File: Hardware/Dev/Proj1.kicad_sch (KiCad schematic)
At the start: 4 parts, among them J1 Conn_01x02, SW1 SW_Push

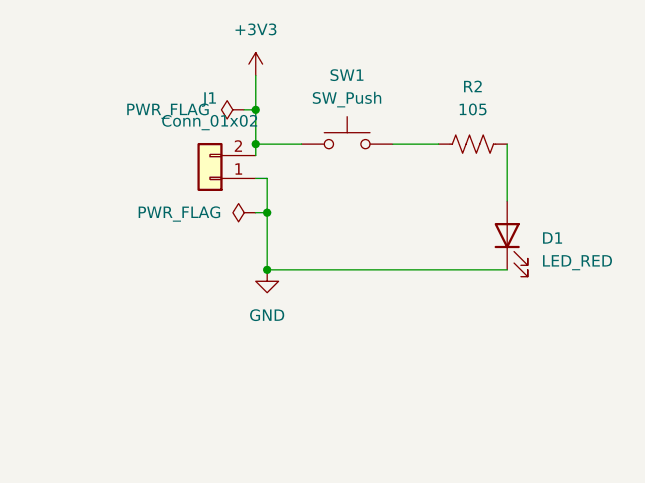
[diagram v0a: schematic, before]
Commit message: onboarding
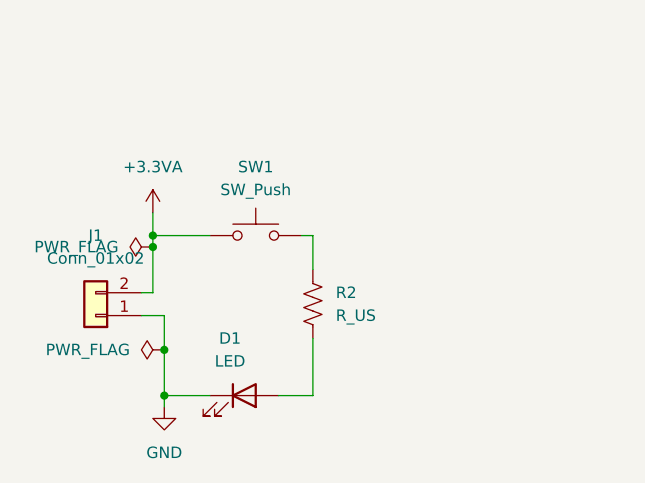
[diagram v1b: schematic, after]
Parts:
- removed R2: 105, Resistor_SMD:R_0603_1608Metric_Pad0.98x0.95mm_HandSolder, symbol Device:R_US
- added R2: R_US, symbol device:R_US
- D1: value LED_RED -> LED; Notes (none) -> (none)
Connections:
- net at SW1.2: now also R2.1
- net at D1.2 (A): now also R2.2
- net +3V3 renamed +3.3VA
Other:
- title: LED Project  -> LED Project
